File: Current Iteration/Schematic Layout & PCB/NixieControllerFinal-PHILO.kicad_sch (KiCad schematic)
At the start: 91 parts, among them J1 Conn_01x10_Pin, J2 USB_C_Receptacle_2.0, J3 Conn_01x10_Pin, J4 Conn_01x10_Pin, J5 Conn_01x10_Pin, J6 Conn_01x02, J7 Micro_SD_Card_Det1, J8 Conn_ARM_JTAG_SWD_10, J9 NixieIN, SW1 PEC11J-9215F-S0015, SW5 PEC16-2015F-N0024, SW6 PEC16-2015F-N0024, U1 HV5622PG, U10 NID1100, U11 TPS61040DBV, U13 STM32G0B1KEU6, U14 CM1224-04MR, U2 HV5622PG, U3 4504, U4 CM1224-04MR, U5 NCH6100HV, U6 CAP1206-x-SL, U7 NID1100, U8 MCP1700x-330xxTT, U9 MAX98357A

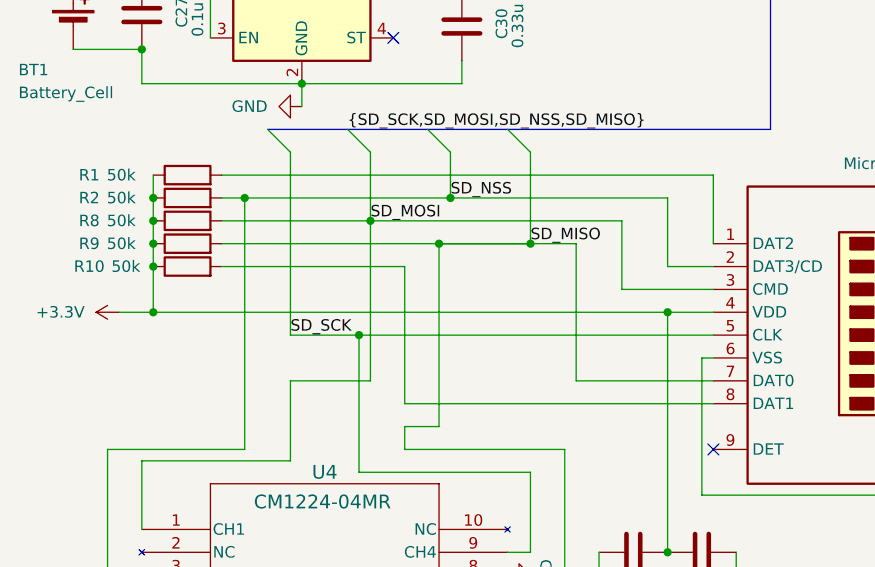
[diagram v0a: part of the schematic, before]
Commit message: Working SPI protocol, SD reading, OS development
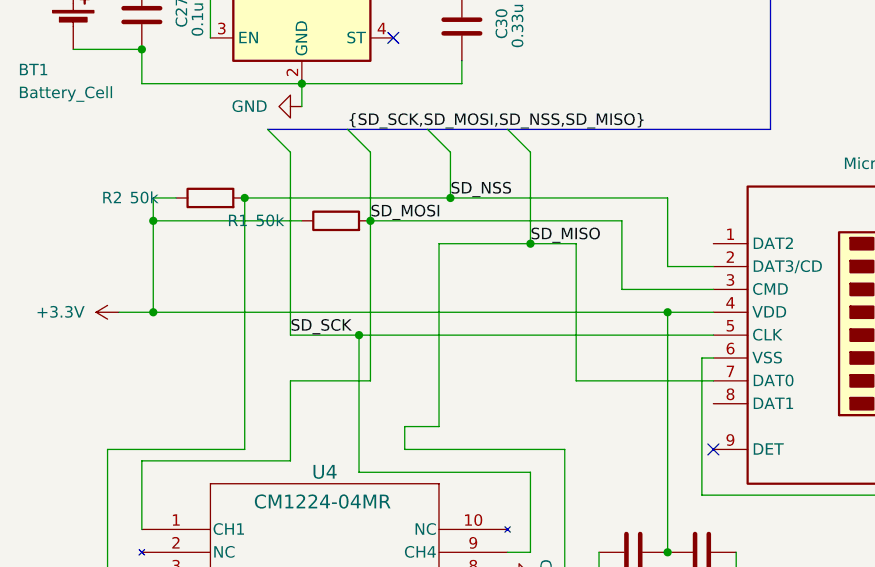
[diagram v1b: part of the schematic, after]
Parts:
- removed R10, R8, R9: 50k, Resistor_SMD:R_0805_2012Metric_Pad1.20x1.40mm_HandSolder, symbol Device:R
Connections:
- net SD_MOSI: now also R1.2
- net at J7.1 (DAT2): no longer R1.2
